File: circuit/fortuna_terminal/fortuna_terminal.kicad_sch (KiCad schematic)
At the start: 11 parts

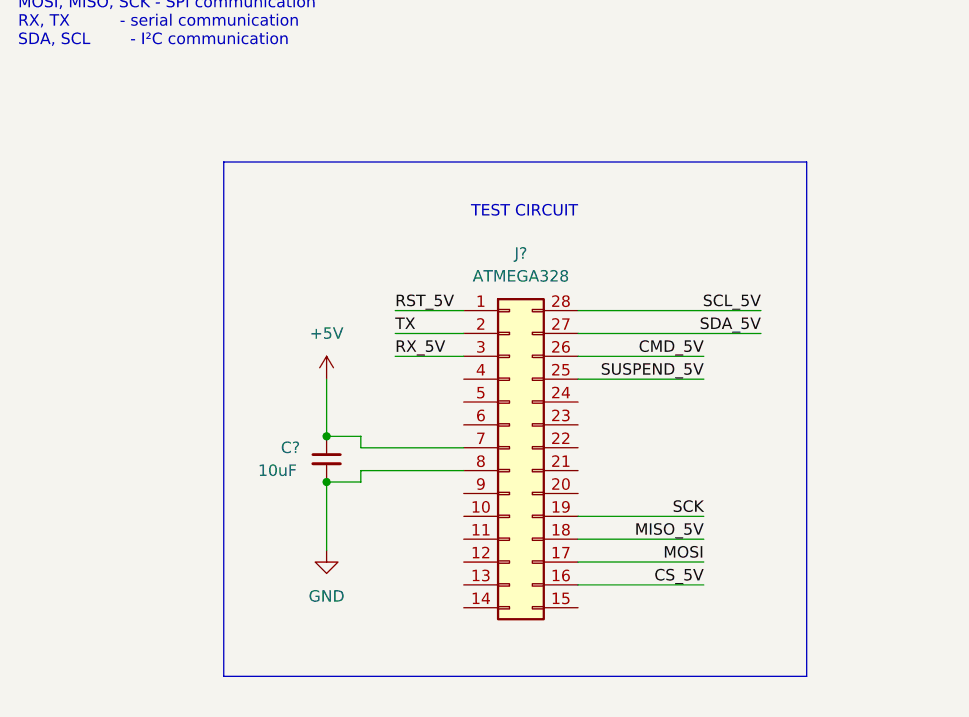
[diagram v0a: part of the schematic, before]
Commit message: .
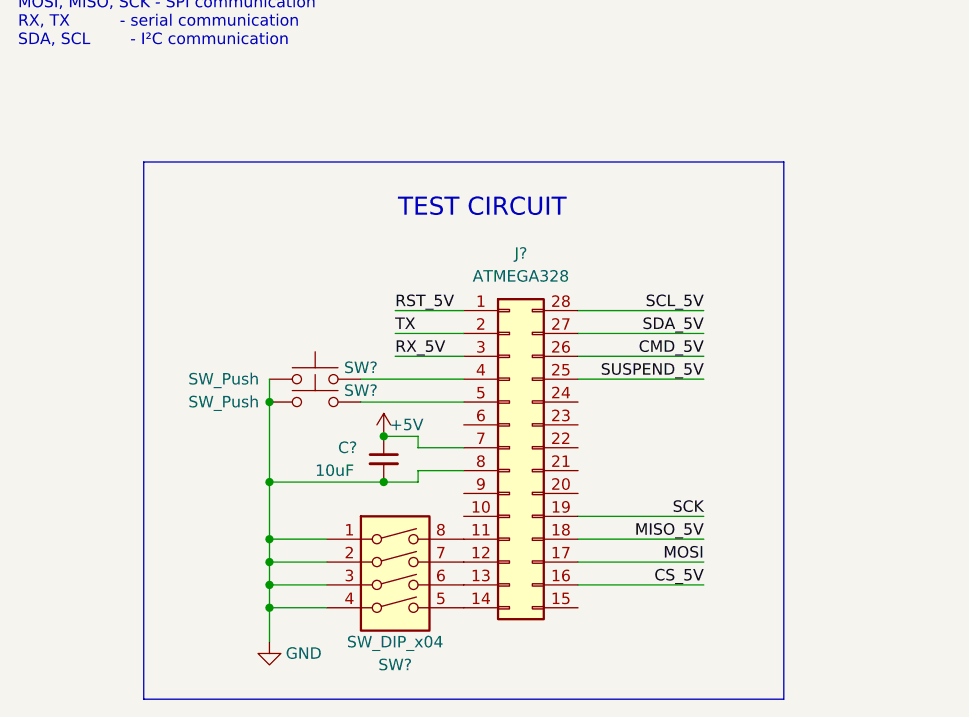
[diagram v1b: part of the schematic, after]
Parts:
- added SW?: SW_DIP_x04, symbol Switch:SW_DIP_x04
- added SW? (x2): SW_Push, symbol Switch:SW_Push
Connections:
- net GND: now also SW?.1, SW?.1, SW?.1, SW?.2, SW?.3, SW?.4
- net at J?.11 (Pin_11): now also SW?.8
- net at J?.12 (Pin_12): now also SW?.7
- net at J?.13 (Pin_13): now also SW?.6
- net at J?.14 (Pin_14): now also SW?.5
- net at J?.4 (Pin_4): now also SW?.2
- net at J?.5 (Pin_5): now also SW?.2
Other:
- moved on the sheet: C?
